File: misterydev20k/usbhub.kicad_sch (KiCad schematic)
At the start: 21 parts, among them J10 USB_A, J7 USB_A, J8 USB_A, J9 USB_A, U7 CH334U, Y3 12MHz

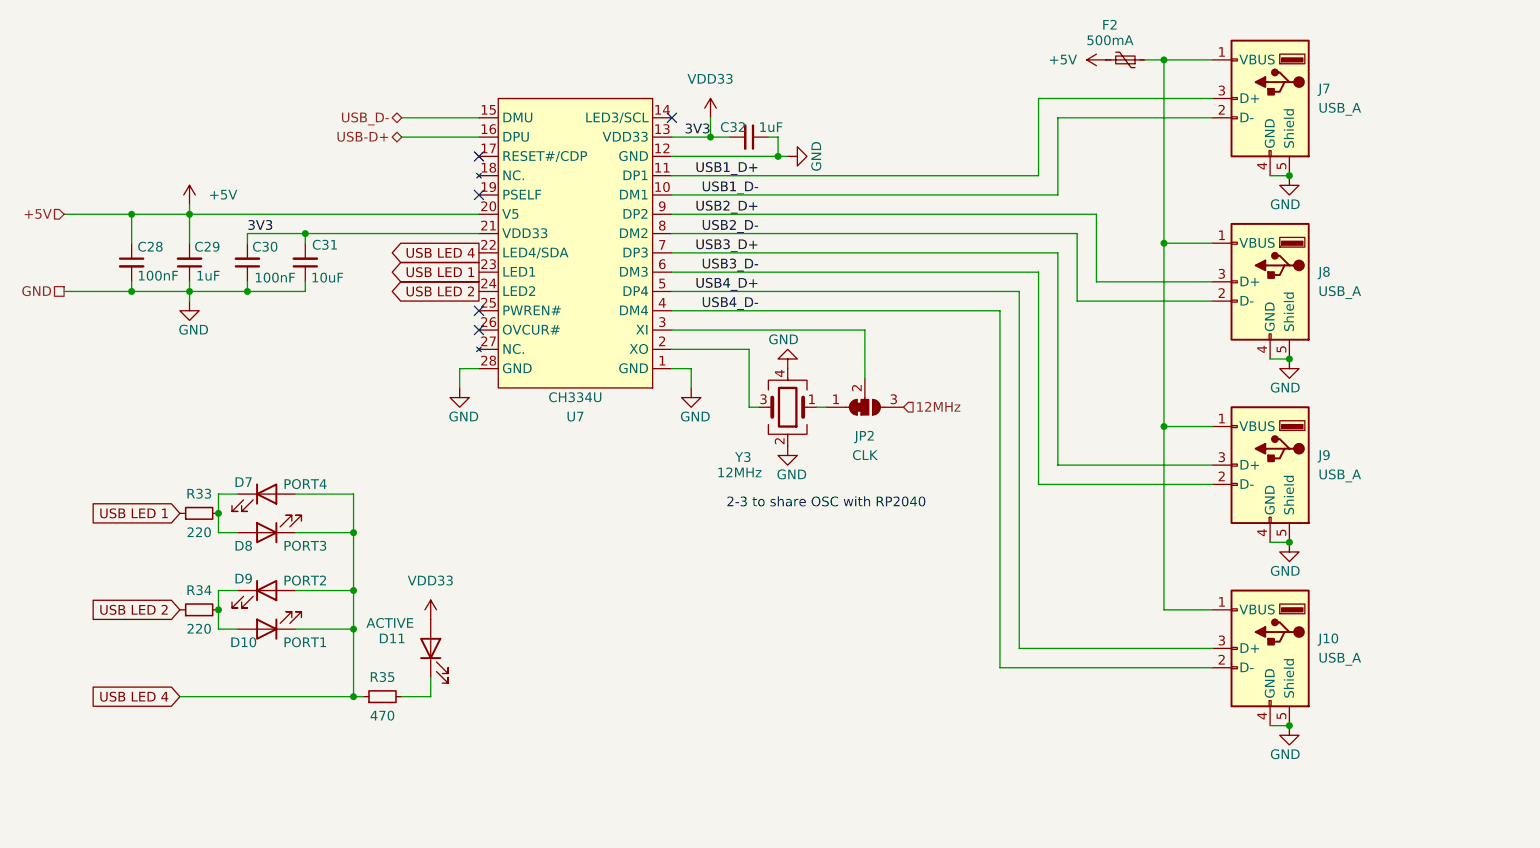
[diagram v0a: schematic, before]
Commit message: More updates in dev20k
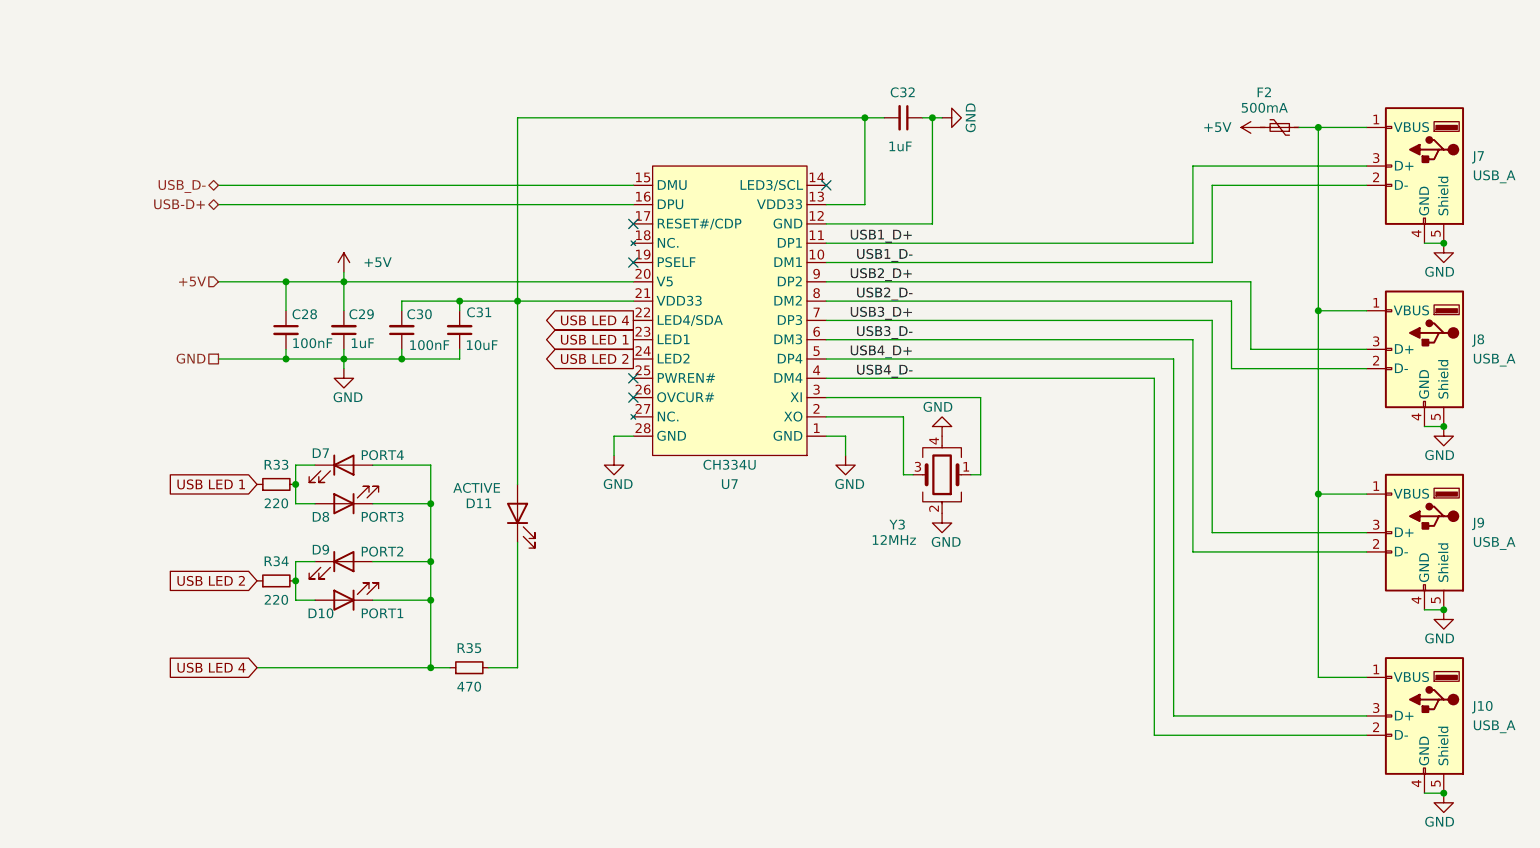
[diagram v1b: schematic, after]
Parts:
- removed JP2: CLK, Jumper:SolderJumper-3_P1.3mm_Bridged12_RoundedPad1.0x1.5mm, symbol Jumper:SolderJumper_3_Bridged12
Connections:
- net at U7.3 (XI): now also Y3.1
- net VDD33: no longer names the net of C30.2, C31.2, C32.2, D11.2 (A), U7.13 (VDD33), U7.21 (VDD33)
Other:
- note removed: "2-3 to share OSC with RP2040"
- moved on the sheet: C28, C29, C30, C31, C32, D10, D11, D7, D8, D9, F2, J10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

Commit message: Update board
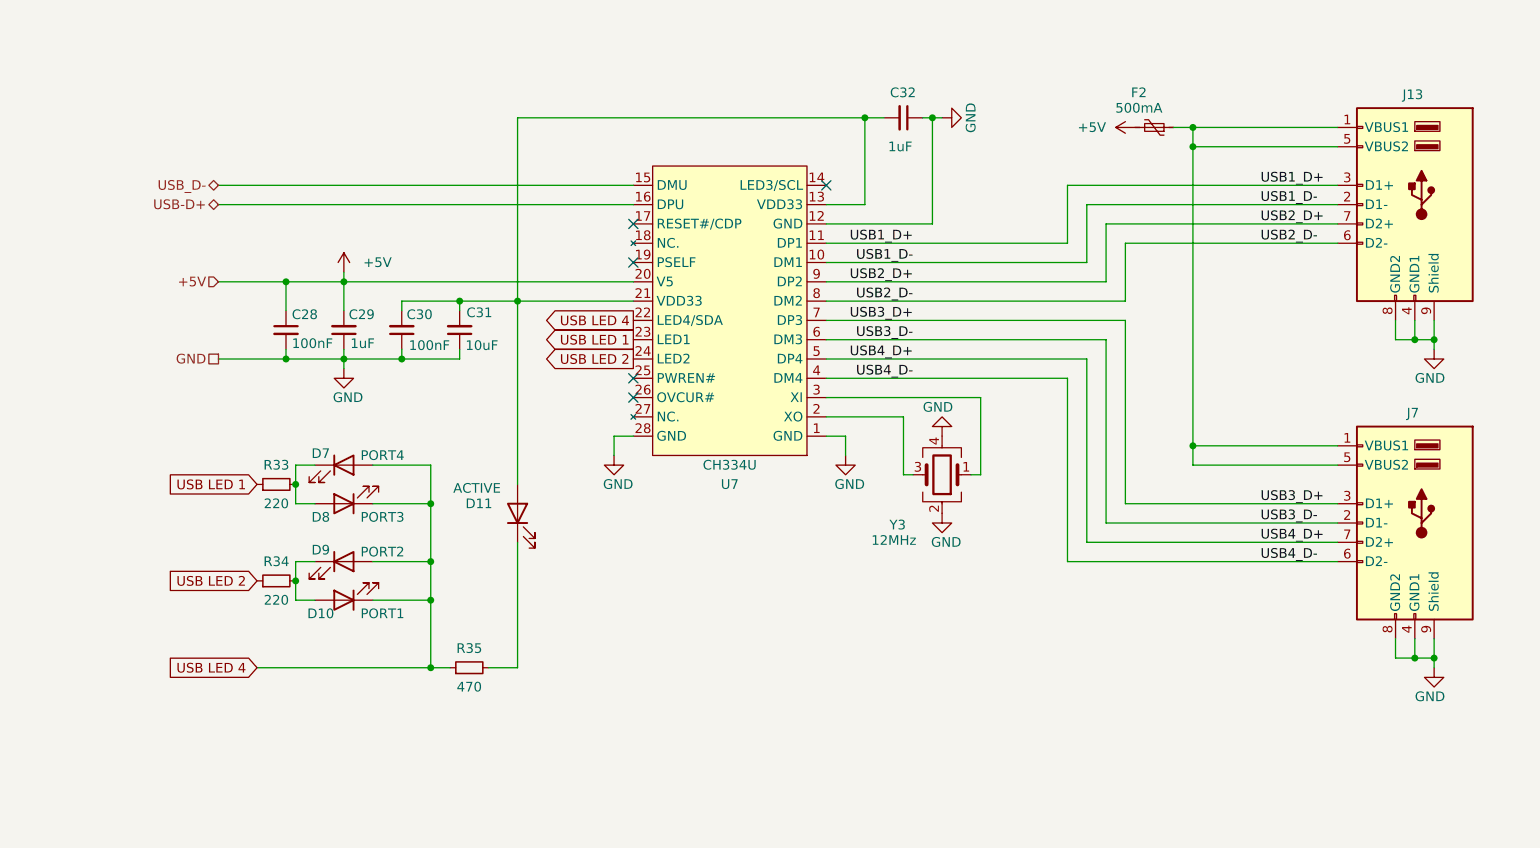
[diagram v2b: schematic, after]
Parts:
- removed J10, J7, J8, J9: USB_A, Connector_USB:USB_A_Molex_67643_Horizontal, symbol Connector:USB_A
- added J13, J7: USB_A_Stacked, Connector_USB:USB_A_Wuerth_61400826021_Horizontal_Stacked, symbol misteryshield20kpico:USB_A_Stacked
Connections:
- net GND: now also J13.4 (GND1), J13.8 (GND2), J13.9 (Shield), J7.4 (GND1), J7.8 (GND2), J7.9 (Shield)
- net USB1_D+: now also J13.3 (D1+)
- net USB1_D-: now also J13.2 (D1-)
- net USB2_D+: now also J13.7 (D2+)
- net USB2_D-: now also J13.6 (D2-)
- net USB3_D+: now also J7.3 (D1+)
- net USB3_D-: now also J7.2 (D1-)
- net USB4_D+: now also J7.7 (D2+)
- net USB4_D-: now also J7.6 (D2-)
- net at F2.1: now also J13.1 (VBUS1), J13.5 (VBUS2), J7.1 (VBUS1), J7.5 (VBUS2)
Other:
- moved on the sheet: F2
